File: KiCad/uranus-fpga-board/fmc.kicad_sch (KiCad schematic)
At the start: 51 parts, among them J1 ASP-134486-01, Q1 2N7002, U10 TLV6700DDCR, U11 TLV6700DDCR, U12 TMUX1108PW, U13 TLV6700DDCR, U6 TPS2553DBVR, U7 SY6288F1ABC, U8 SY6874DBC, U9 TLV6700DDCR

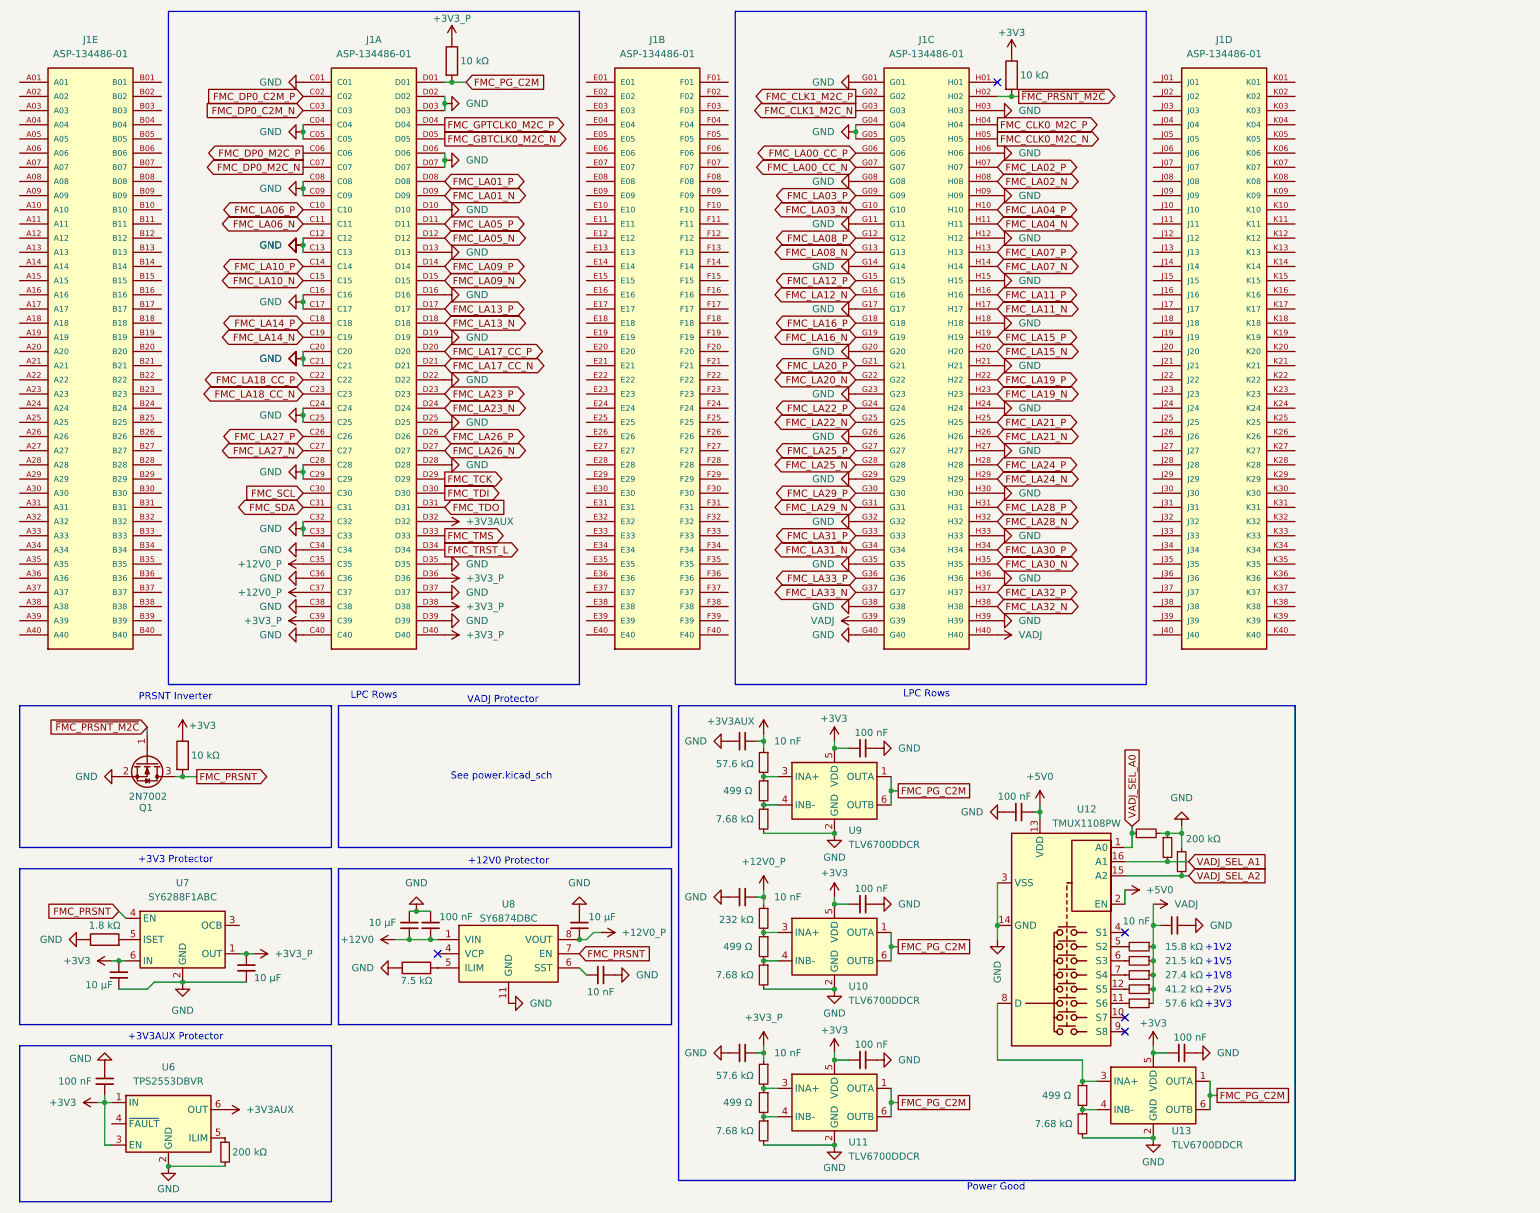
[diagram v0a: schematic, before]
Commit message: big things happening in schematic quality
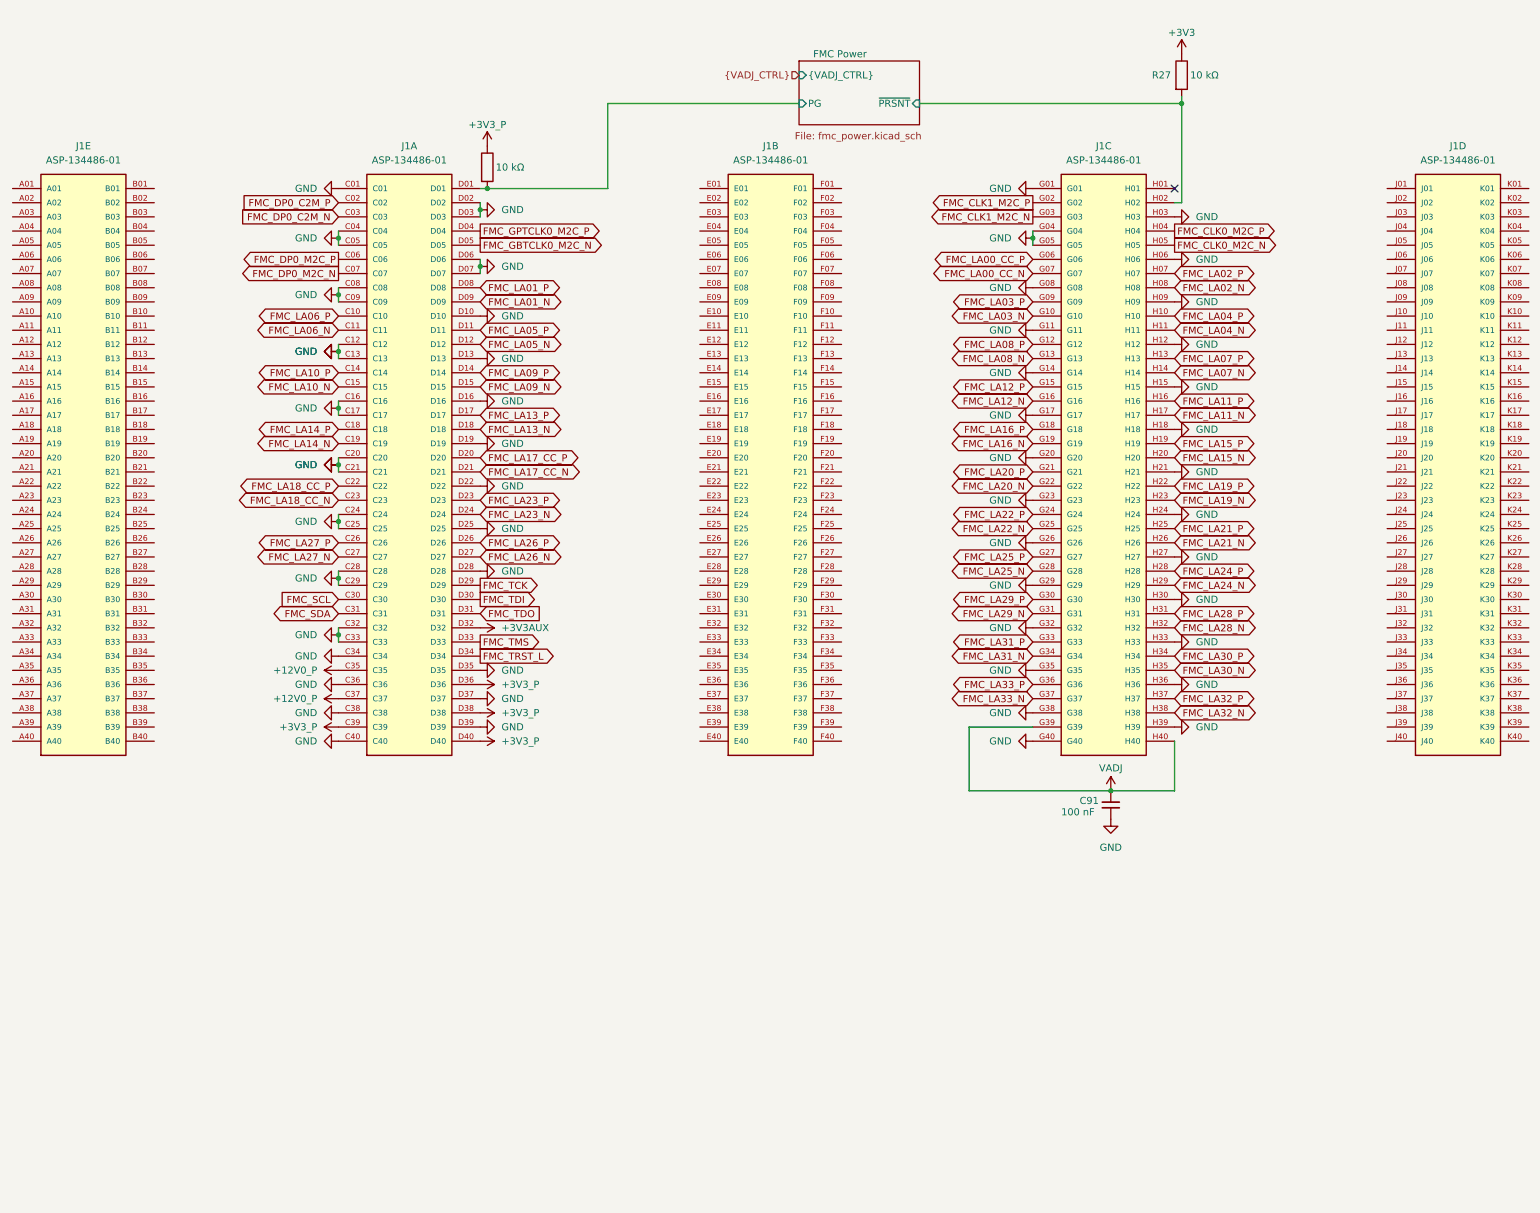
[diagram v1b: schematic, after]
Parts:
- removed C70, C74, C80, C81, C82, C83, C85: 100 nF, symbol Device:C_Small
- removed C71, C72, C73, C75: 10 μF, symbol Device:C_Small
- removed C76, C77, C78, C79, C84: 10 nF, symbol Device:C_Small
- removed Q1: 2N7002, Package_TO_SOT_SMD:SOT-23, symbol Transistor_FET:2N7002
- removed R13: 1.8 kΩ, Resistor_SMD:R_0402_1005Metric, symbol Device:R
- removed R14: 10 kΩ, Resistor_SMD:R_0201_0603Metric, symbol Device:R
- removed R15: 200 kΩ, Resistor_SMD:R_0402_1005Metric, symbol Device:R_Small
- removed R16: 7.5 kΩ, Resistor_SMD:R_0201_0603Metric, symbol Device:R
- removed R18, R24, R34: 57.6 kΩ, Resistor_SMD:R_0402_1005Metric, symbol Device:R_Small
- removed R19, R22, R25, R28: 499 Ω, Resistor_SMD:R_0201_0603Metric, symbol Device:R_Small
- removed R20, R23, R26, R29: 7.68 kΩ, Resistor_SMD:R_0402_1005Metric, symbol Device:R_Small
- removed R21: 232 kΩ, Resistor_SMD:R_0402_1005Metric, symbol Device:R_Small
- removed R30: 15.8 kΩ, Resistor_SMD:R_0402_1005Metric, symbol Device:R_Small
- removed R31: 21.5 kΩ, Resistor_SMD:R_0402_1005Metric, symbol Device:R_Small
- removed R32: 27.4 kΩ, Resistor_SMD:R_0402_1005Metric, symbol Device:R_Small
- removed R33: 41.2 kΩ, Resistor_SMD:R_0402_1005Metric, symbol Device:R_Small
- removed R35, R36, R37: 200 kΩ, Resistor_SMD:R_0201_0603Metric, symbol Device:R_Small
- removed U10, U11, U13, U9: TLV6700DDCR, Package_TO_SOT_SMD:SOT-23-6, symbol Sensor_Touch:AT42QT1011-TSHR
- removed U12: TMUX1108PW, Package_SO:TSSOP-16_4.4x5mm_P0.65mm, symbol Analog_Switch:TMUX1108PW
- removed U6: TPS2553DBVR, Package_TO_SOT_SMD:SOT-23-6, symbol Battery_Management:BQ21040DBV
- removed U7: SY6288F1ABC, Package_TO_SOT_SMD:SOT-23-6, symbol Power_Management:AP2171W
- removed U8: SY6874DBC, Package_DFN_QFN:DFN-10-1EP_3x3mm_P0.5mm_EP1.75x2.7mm, symbol Connector_Generic:Conn_02x05_Counter_Clockwise
- added C91: 100 nF, symbol Device:C_Small
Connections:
- net GND: now also C91.2
- net VADJ: now also C91.1
- net FMC_PG_C2M renamed FMC Power/PG
- net ~{FMC_PRSNT_M2C} renamed FMC Power/~{PRSNT}
- no-connect marks 5 -> 1
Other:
- added sheet FMC Power (fmc_power.kicad_sch)
- note removed: "+12V0 Protector"
- note removed: "+1V2"
- note removed: "+1V5"
- note removed: "+1V8"
- note removed: "+2V5"
- note removed: "+3V3"
- note removed: "+3V3 Protector"
- note removed: "+3V3AUX Protector"
- note removed: "LPC Rows"
- note removed: "PRSNT Inverter"
- note removed: "Power Good"
- note removed: "See power.kicad_sch"
- note removed: "VADJ Protector"
- moved on the sheet: J1A, J1B, J1C, J1D, J1E

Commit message: Big things have mostly happened in schematic quality
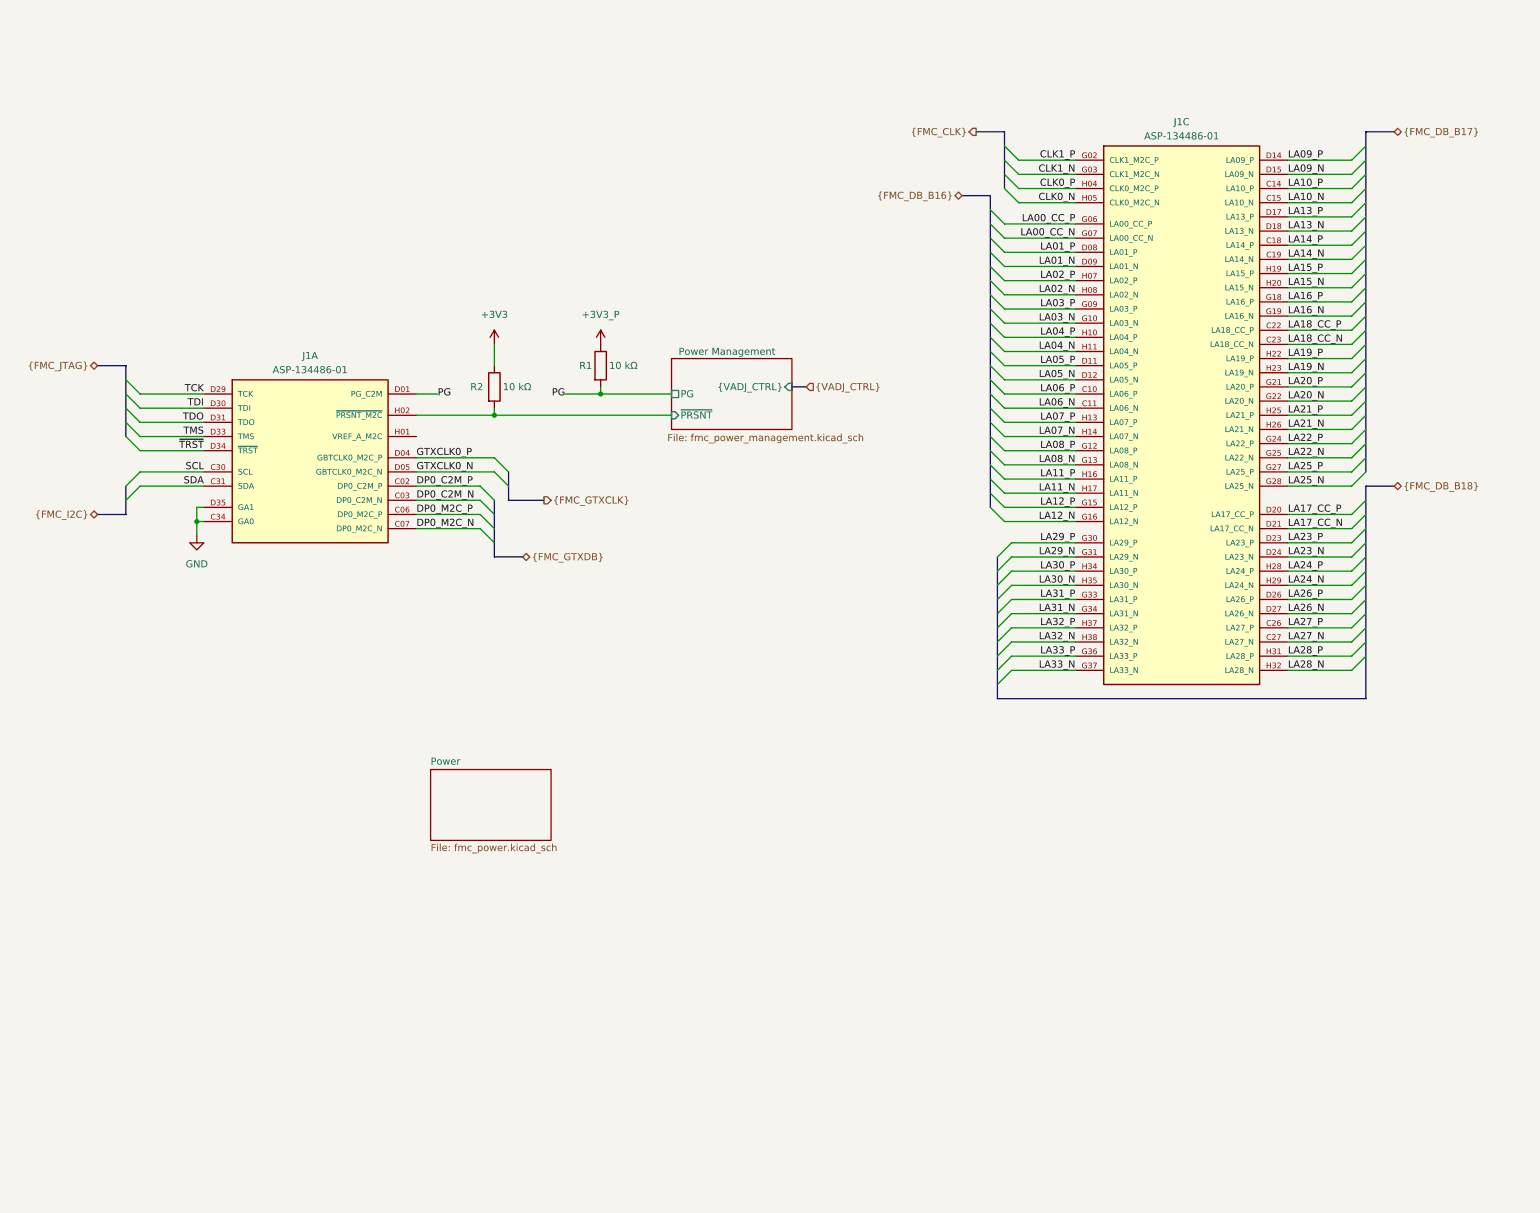
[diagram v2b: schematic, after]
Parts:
- removed C91: 100 nF, symbol Device:C_Small
- removed unit 2 of J1
- removed unit 5 of J1
- removed unit 4 of J1
- renumbered R17 to R1, R27 to R2
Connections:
- net +3V3_P: no longer J1.C39, J1.D36, J1.D38, J1.D40
- net Power Management/~{PRSNT}: now also J1.H02 (~{PRSNT_M2C}); no longer J1.H02
- net GND: no longer J1.C01, J1.C04, J1.C05, J1.C08, J1.C09, J1.C12, J1.C13, J1.C16, J1.C17, J1.C20, J1.C21, J1.C24, J1.C25, J1.C28, J1.C29, J1.C32, J1.C33, J1.C36, J1.C38, J1.C40, J1.D02, J1.D03, J1.D06, J1.D07, J1.D10, J1.D13, J1.D16, J1.D19, J1.D22, J1.D25, J1.D28, J1.D37, J1.D39, J1.G01, J1.G04, J1.G05, J1.G08, J1.G11, J1.G14, J1.G17, J1.G20, J1.G23, J1.G26, J1.G29, J1.G32, J1.G35, J1.G38, J1.G40, J1.H03, J1.H06, J1.H09, J1.H12, J1.H15, J1.H18, J1.H21, J1.H24, J1.H27, J1.H30, J1.H33, J1.H36, J1.H39
- removed net +12V0_P: J1.C35, J1.C37
- removed net +3V3AUX: J1.D32
- net Power Management/PG renamed PG
- net FMC_CLK0_M2C_N renamed CLK0_N
- net FMC_CLK0_M2C_P renamed CLK0_P
- net FMC_CLK1_M2C_N renamed CLK1_N
- net FMC_CLK1_M2C_P renamed CLK1_P
- net FMC_DP0_C2M_N renamed DP0_C2M_N
- net FMC_DP0_C2M_P renamed DP0_C2M_P
- net FMC_DP0_M2C_N renamed DP0_M2C_N
- net FMC_DP0_M2C_P renamed DP0_M2C_P
- net FMC_GBTCLK0_M2C_N renamed GTXCLK0_N
- net FMC_GPTCLK0_M2C_P renamed GTXCLK0_P
- net FMC_LA00_CC_N renamed LA00_CC_N
- net FMC_LA00_CC_P renamed LA00_CC_P
- removed net FMC_LA01_N: J1.D09
- removed net FMC_LA01_P: J1.D08
- net FMC_LA02_N renamed LA02_N
- net FMC_LA02_P renamed LA02_P
- net FMC_LA03_N renamed LA03_N
- net FMC_LA03_P renamed LA03_P
- net FMC_LA04_N renamed LA04_N
- net FMC_LA04_P renamed LA04_P
- removed net FMC_LA05_N: J1.D12
- removed net FMC_LA05_P: J1.D11
- removed net FMC_LA06_N: J1.C11
- removed net FMC_LA06_P: J1.C10
- net FMC_LA07_N renamed LA07_N
- net FMC_LA07_P renamed LA07_P
- net FMC_LA08_N renamed LA08_N
- net FMC_LA08_P renamed LA08_P
- removed net FMC_LA09_N: J1.D15
- removed net FMC_LA09_P: J1.D14
- removed net FMC_LA10_N: J1.C15
- removed net FMC_LA10_P: J1.C14
- net FMC_LA11_N renamed LA11_N
- net FMC_LA11_P renamed LA11_P
- net FMC_LA12_N renamed LA12_N
- net FMC_LA12_P renamed LA12_P
- removed net FMC_LA13_N: J1.D18
- removed net FMC_LA13_P: J1.D17
- removed net FMC_LA14_N: J1.C19
- removed net FMC_LA14_P: J1.C18
- net FMC_LA15_N renamed LA15_N
- net FMC_LA15_P renamed LA15_P
- net FMC_LA16_N renamed LA16_N
- net FMC_LA16_P renamed LA16_P
- removed net FMC_LA17_CC_N: J1.D21
- removed net FMC_LA17_CC_P: J1.D20
- removed net FMC_LA18_CC_N: J1.C23
- removed net FMC_LA18_CC_P: J1.C22
- net FMC_LA19_N renamed LA19_N
- net FMC_LA19_P renamed LA19_P
- net FMC_LA20_N renamed LA20_N
- net FMC_LA20_P renamed LA20_P
- net FMC_LA21_N renamed LA21_N
- net FMC_LA21_P renamed LA21_P
- net FMC_LA22_N renamed LA22_N
- net FMC_LA22_P renamed LA22_P
- removed net FMC_LA23_N: J1.D24
- removed net FMC_LA23_P: J1.D23
- net FMC_LA24_N renamed LA24_N
- net FMC_LA24_P renamed LA24_P
- net FMC_LA25_N renamed LA25_N
- net FMC_LA25_P renamed LA25_P
- removed net FMC_LA26_N: J1.D27
- removed net FMC_LA26_P: J1.D26
- removed net FMC_LA27_N: J1.C27
- removed net FMC_LA27_P: J1.C26
- net FMC_LA28_N renamed LA28_N
- net FMC_LA28_P renamed LA28_P
- net FMC_LA29_N renamed LA29_N
- net FMC_LA29_P renamed LA29_P
- net FMC_LA30_N renamed LA30_N
- net FMC_LA30_P renamed LA30_P
- net FMC_LA31_N renamed LA31_N
- net FMC_LA31_P renamed LA31_P
- net FMC_LA32_N renamed LA32_N
- net FMC_LA32_P renamed LA32_P
- net FMC_LA33_N renamed LA33_N
- net FMC_LA33_P renamed LA33_P
- net FMC_SCL renamed SCL
- net FMC_SDA renamed SDA
- net FMC_TCK renamed TCK
- net FMC_TDI renamed TDI
- net FMC_TDO renamed TDO
- net FMC_TMS renamed TMS
- net FMC_TRST_L renamed ~{TRST}
- removed net VADJ: J1.G39, J1.H40
- new net LA01_N: J1.D09 (LA01_N)
- new net LA01_P: J1.D08 (LA01_P)
- new net LA05_N: J1.D12 (LA05_N)
- new net LA05_P: J1.D11 (LA05_P)
- new net LA06_N: J1.C11 (LA06_N)
- new net LA06_P: J1.C10 (LA06_P)
- new net LA09_N: J1.D15 (LA09_N)
- new net LA09_P: J1.D14 (LA09_P)
- new net LA10_N: J1.C15 (LA10_N)
- new net LA10_P: J1.C14 (LA10_P)
- new net LA13_N: J1.D18 (LA13_N)
- new net LA13_P: J1.D17 (LA13_P)
- new net LA14_N: J1.C19 (LA14_N)
- new net LA14_P: J1.C18 (LA14_P)
- new net LA17_CC_N: J1.D21 (LA17_CC_N)
- new net LA17_CC_P: J1.D20 (LA17_CC_P)
- new net LA18_CC_N: J1.C23 (LA18_CC_N)
- new net LA18_CC_P: J1.C22 (LA18_CC_P)
- new net LA23_N: J1.D24 (LA23_N)
- new net LA23_P: J1.D23 (LA23_P)
- new net LA26_N: J1.D27 (LA26_N)
- new net LA26_P: J1.D26 (LA26_P)
- new net LA27_N: J1.C27 (LA27_N)
- new net LA27_P: J1.C26 (LA27_P)
- no-connect marks 1 -> 0
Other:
- sheet FMC Power renamed Power Management
- added sheet Power (fmc_power.kicad_sch)
- sheet Power Management: file fmc_power.kicad_sch -> fmc_power_management.kicad_sch
- moved on the sheet: R2
